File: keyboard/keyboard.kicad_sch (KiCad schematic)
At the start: 157 parts, among them SW1 SW_Push, SW10 SW_Push, SW11 SW_Push, SW12 SW_Push, SW13 SW_Push, SW14 SW_Push, SW15 SW_Push, SW16 SW_Push, SW17 SW_Push, SW18 SW_Push, SW19 SW_Push, SW2 SW_Push, SW20 SW_Push, SW21 SW_Push, SW22 SW_Push, SW23 SW_Push, SW24 SW_Push, SW25 SW_Push, SW26 SW_Push, SW27 SW_Push, SW28 SW_Push, SW29 SW_Push, SW3 SW_Push, SW30 SW_Push, SW31 SW_Push, SW32 SW_Push, SW33 SW_Push, SW34 SW_Push, SW35 SW_Push, SW36 SW_Push, SW37 SW_Push, SW38 SW_Push, SW39 SW_Push, SW4 SW_Push, SW40 SW_Push, SW41 SW_Push, SW42 SW_Push, SW43 SW_Push, SW44 SW_Push, SW45 SW_Push, SW46 SW_Push, SW47 SW_Push, SW48 SW_Push, SW49 SW_Push, SW5 SW_Push, SW50 SW_Push, SW51 SW_Push, SW52 SW_Push, SW53 SW_Push, SW54 SW_Push, SW55 SW_Push, SW56 SW_Push, SW57 SW_Push, SW58 SW_Push, SW59 SW_Push, SW6 SW_Push, SW60 SW_Push, SW61 SW_Push, SW62 SW_Push, SW63 SW_Push, SW64 SW_Push, SW65 SW_Push, SW66 SW_Push, SW67 SW_Push, SW68 SW_Push, SW69 SW_Push, SW7 SW_Push, SW70 SW_Push, SW71 SW_Push, SW72 SW_Push, SW73 SW_Push, SW74 SW_Push, SW75 SW_Push, SW76 SW_Push, SW77 SW_Push, SW78 SW_Push, SW8 SW_Push, SW9 SW_Push, U1 Pico

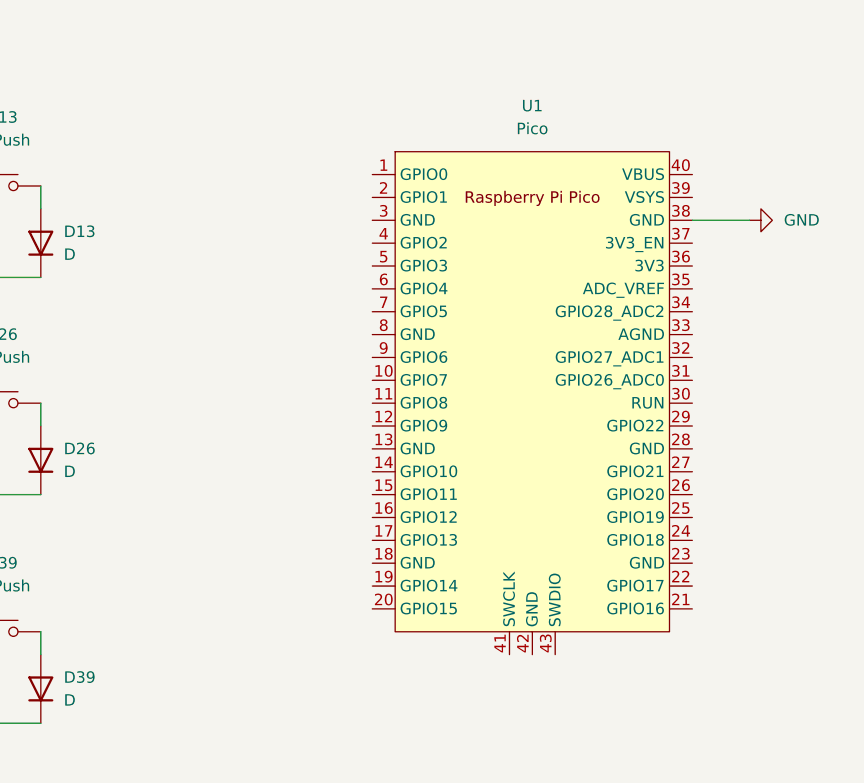
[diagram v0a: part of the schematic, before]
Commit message: saved schematic
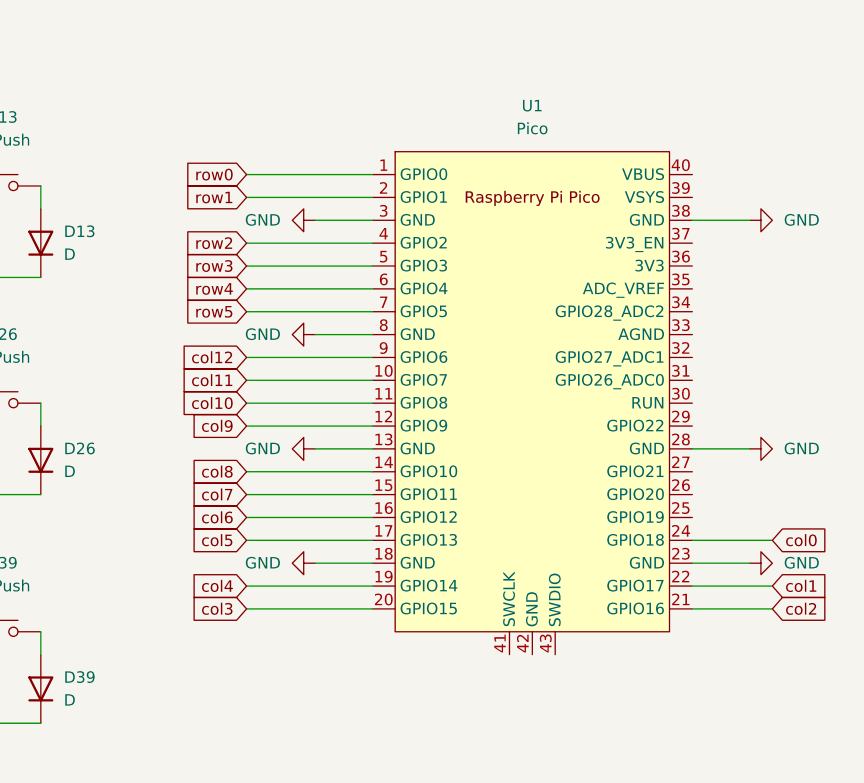
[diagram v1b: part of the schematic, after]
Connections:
- net GND: now also U1.13 (GND), U1.18 (GND), U1.23 (GND), U1.28 (GND), U1.3 (GND), U1.8 (GND)
- net col0: now also U1.24 (GPIO18)
- net col1: now also U1.22 (GPIO17)
- net col10: now also U1.11 (GPIO8)
- net col11: now also U1.10 (GPIO7)
- net col12: now also U1.9 (GPIO6)
- net col2: now also U1.21 (GPIO16)
- net col3: now also U1.20 (GPIO15)
- net col4: now also U1.19 (GPIO14)
- net col5: now also U1.17 (GPIO13)
- net col6: now also U1.16 (GPIO12)
- net col7: now also U1.15 (GPIO11)
- net col8: now also U1.14 (GPIO10)
- net col9: now also U1.12 (GPIO9)
- net row0: now also U1.1 (GPIO0)
- net row1: now also U1.2 (GPIO1)
- net row2: now also U1.4 (GPIO2)
- net row3: now also U1.5 (GPIO3)
- net row4: now also U1.6 (GPIO4)
- net row5: now also U1.7 (GPIO5)
